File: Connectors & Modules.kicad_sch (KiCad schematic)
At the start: 1 part, among them M1 Wireless_Module

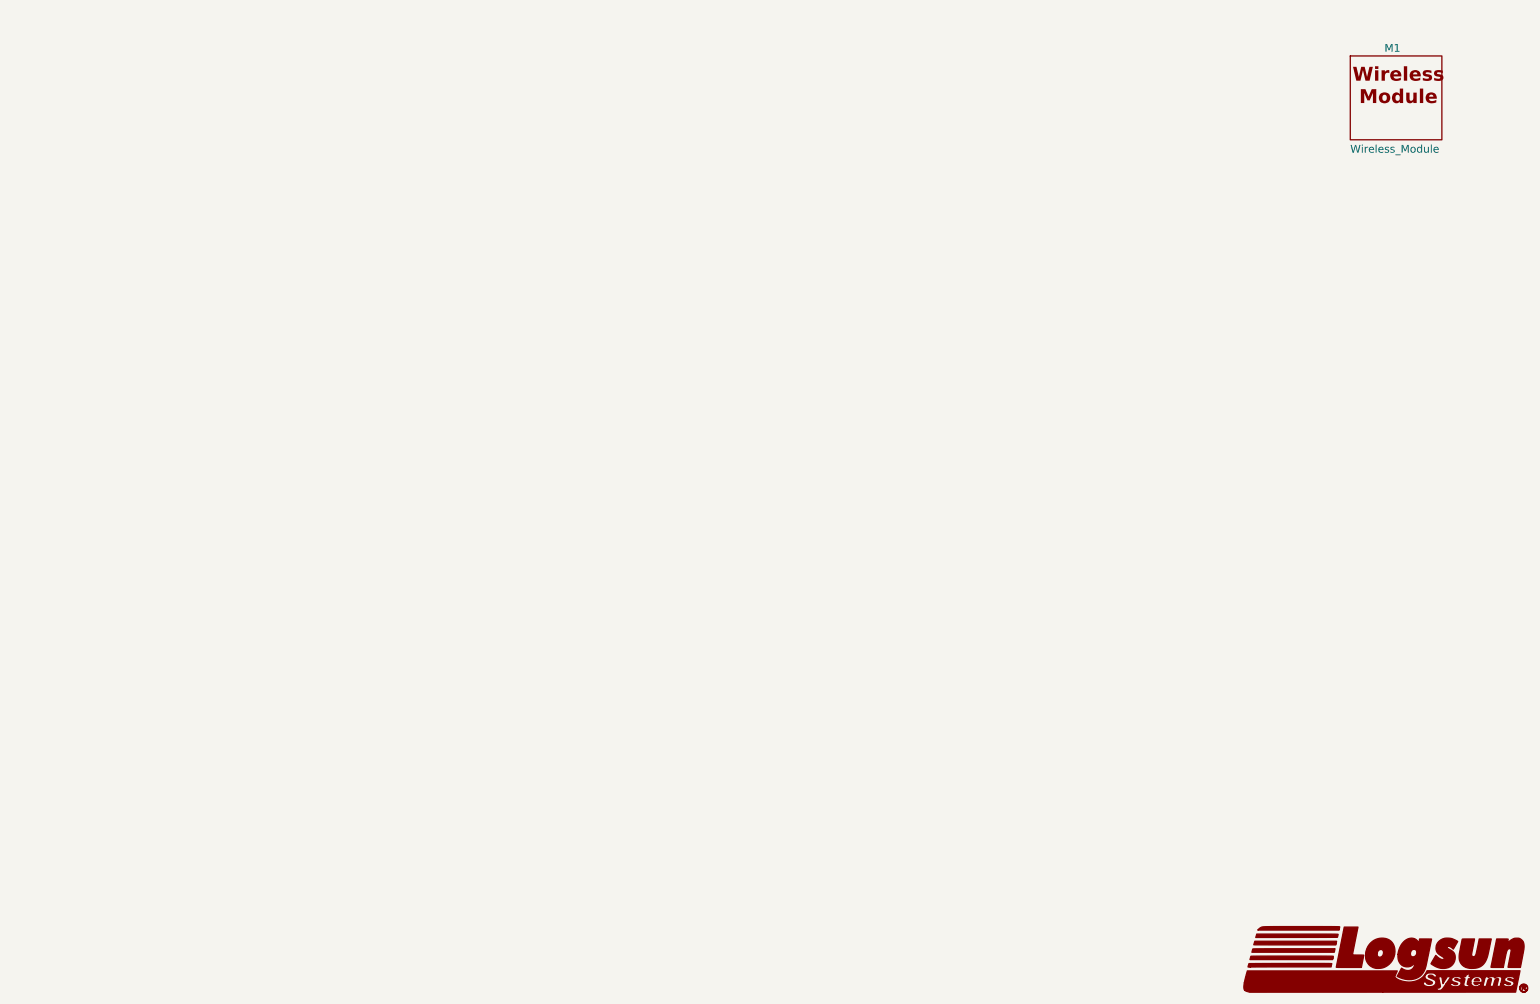
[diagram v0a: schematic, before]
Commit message: Schematic Completed, Footprints Assigned
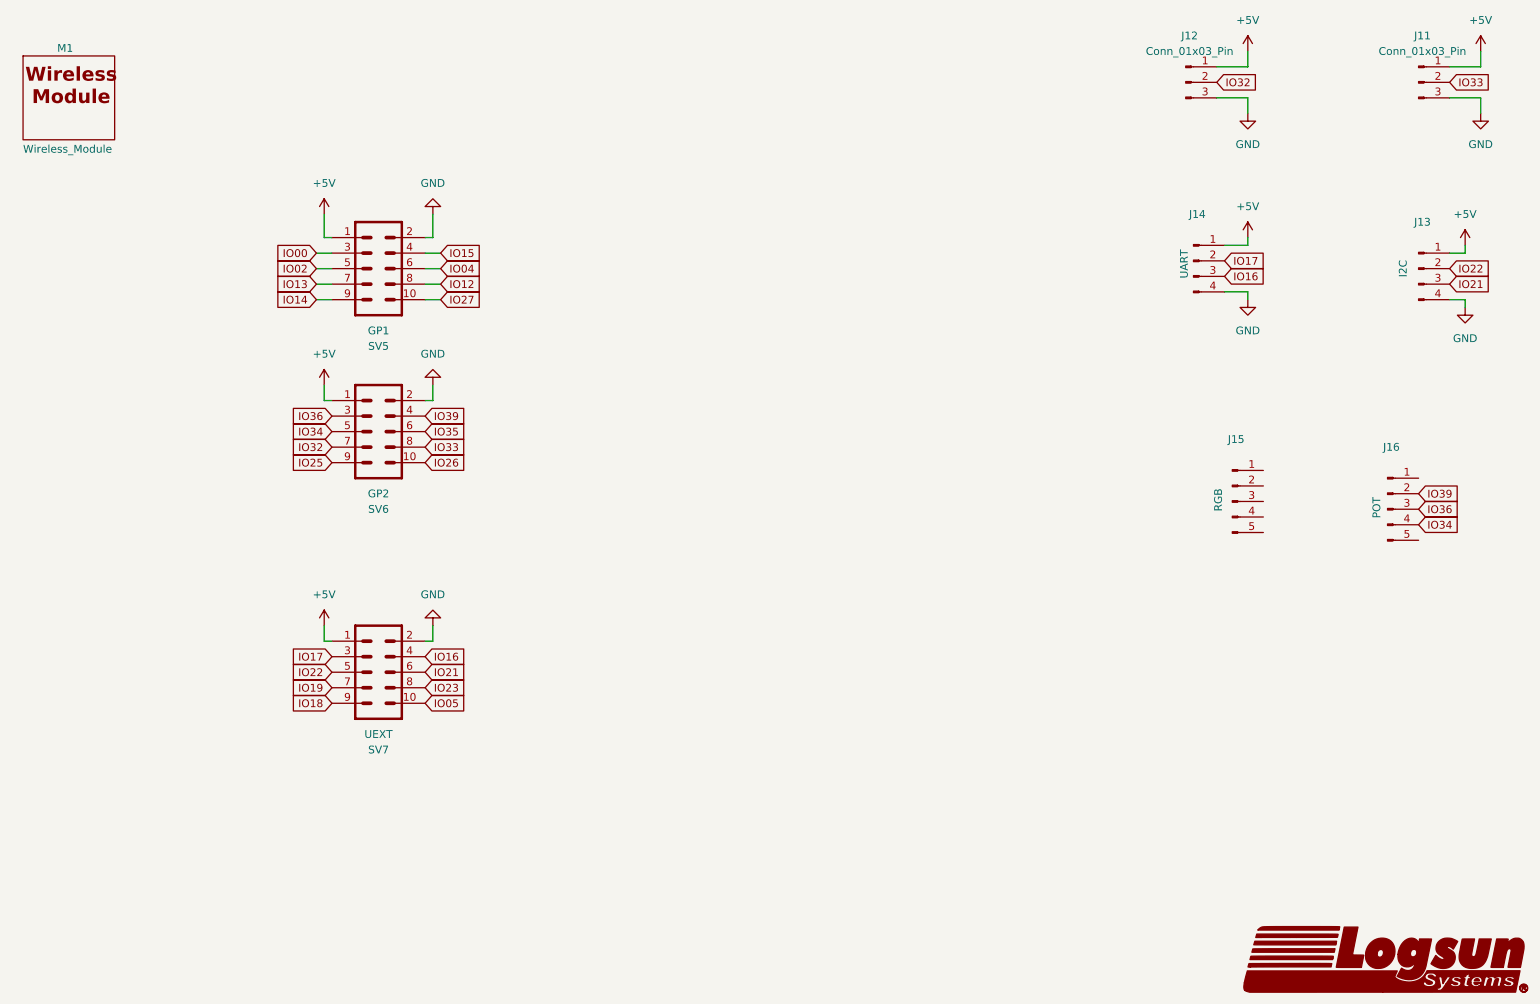
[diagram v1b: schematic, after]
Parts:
- added J11, J12: Conn_01x03_Pin, Connector_JST:JST_EH_B3B-EH-A_1x03_P2.50mm_Vertical, symbol Connector:Conn_01x03_Pin
- added J13: I2C, Connector_JST:JST_EH_B4B-EH-A_1x04_P2.50mm_Vertical, symbol Connector:Conn_01x04_Pin
- added J14: UART, Connector_JST:JST_EH_B4B-EH-A_1x04_P2.50mm_Vertical, symbol Connector:Conn_01x04_Pin
- added J15: RGB, Connector_JST:JST_EH_B5B-EH-A_1x05_P2.50mm_Vertical, symbol Connector:Conn_01x05_Pin
- added J16: POT, Connector_JST:JST_EH_B5B-EH-A_1x05_P2.50mm_Vertical, symbol Connector:Conn_01x05_Pin
- added SV5: GP1, LOGSUN:LGS-KC-ML10-CONTROLLER, symbol LOGSUN:LGS-KC-ML10-CONTROLLER
- added SV6: GP2, LOGSUN:LGS-KC-ML10-CONTROLLER, symbol LOGSUN:LGS-KC-ML10-CONTROLLER
- added SV7: UEXT, LOGSUN:LGS-KC-ML10-CONTROLLER, symbol LOGSUN:LGS-KC-ML10-CONTROLLER
- M1: footprint (none) -> LOGSUN:LGS-KC-Wireless_Mod
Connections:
- new net +5V: J11.1 (Pin_1), J12.1 (Pin_1), J13.1 (Pin_1), J14.1 (Pin_1), SV5.1, SV6.1, SV7.1
- new net GND: J11.3 (Pin_3), J12.3 (Pin_3), J13.4 (Pin_4), J14.4 (Pin_4), SV5.2, SV6.2, SV7.2
- new net IO00: SV5.3
- new net IO02: SV5.5
- new net IO04: SV5.6
- new net IO05: SV7.10
- new net IO12: SV5.8
- new net IO13: SV5.7
- new net IO14: SV5.9
- new net IO15: SV5.4
- new net IO16: J14.3 (Pin_3), SV7.4
- new net IO17: J14.2 (Pin_2), SV7.3
- new net IO18: SV7.9
- new net IO19: SV7.7
- new net IO21: J13.3 (Pin_3), SV7.6
- new net IO22: J13.2 (Pin_2), SV7.5
- new net IO23: SV7.8
- new net IO25: SV6.9
- new net IO26: SV6.10
- new net IO27: SV5.10
- new net IO32: J12.2 (Pin_2), SV6.7
- new net IO33: J11.2 (Pin_2), SV6.8
- new net IO34: J16.4 (Pin_4), SV6.5
- new net IO35: SV6.6
- new net IO36: J16.3 (Pin_3), SV6.3
- new net IO39: J16.2 (Pin_2), SV6.4
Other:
- moved on the sheet: M1
